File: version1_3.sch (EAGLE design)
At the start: 70 parts, among them U1 LIGHTSA, U2 LIGHTSB, U3 ButtonB, U4 ButtonA

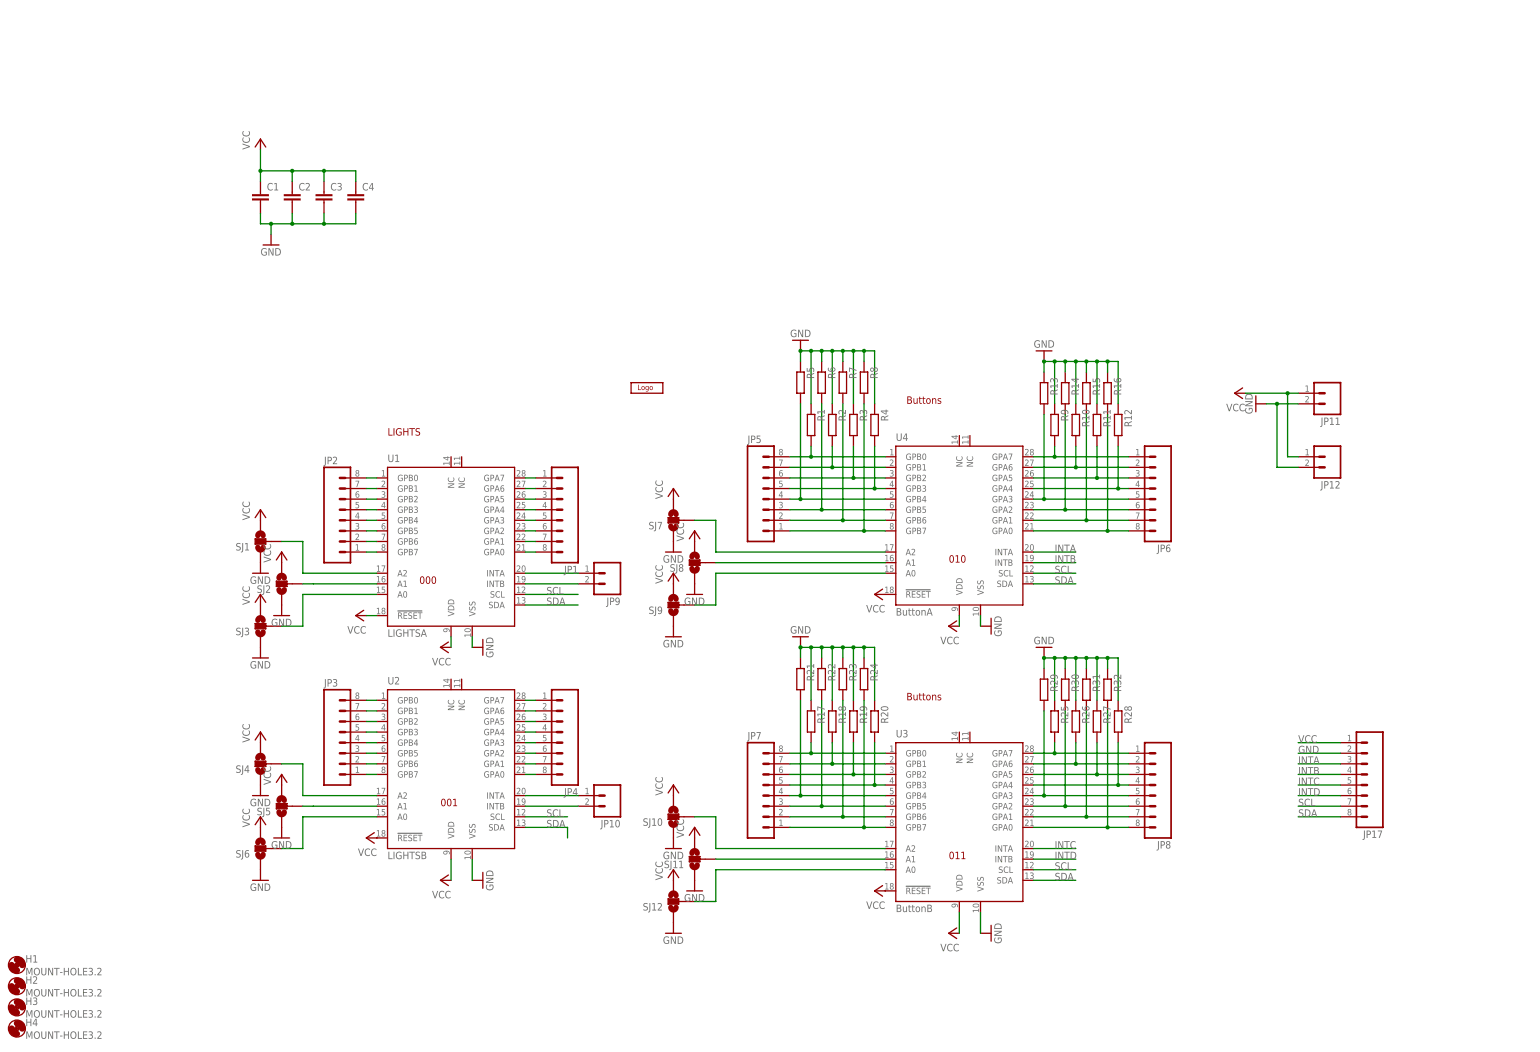
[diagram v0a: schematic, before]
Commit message: folder cleanup and added pdfs and pngs of schematic and layout
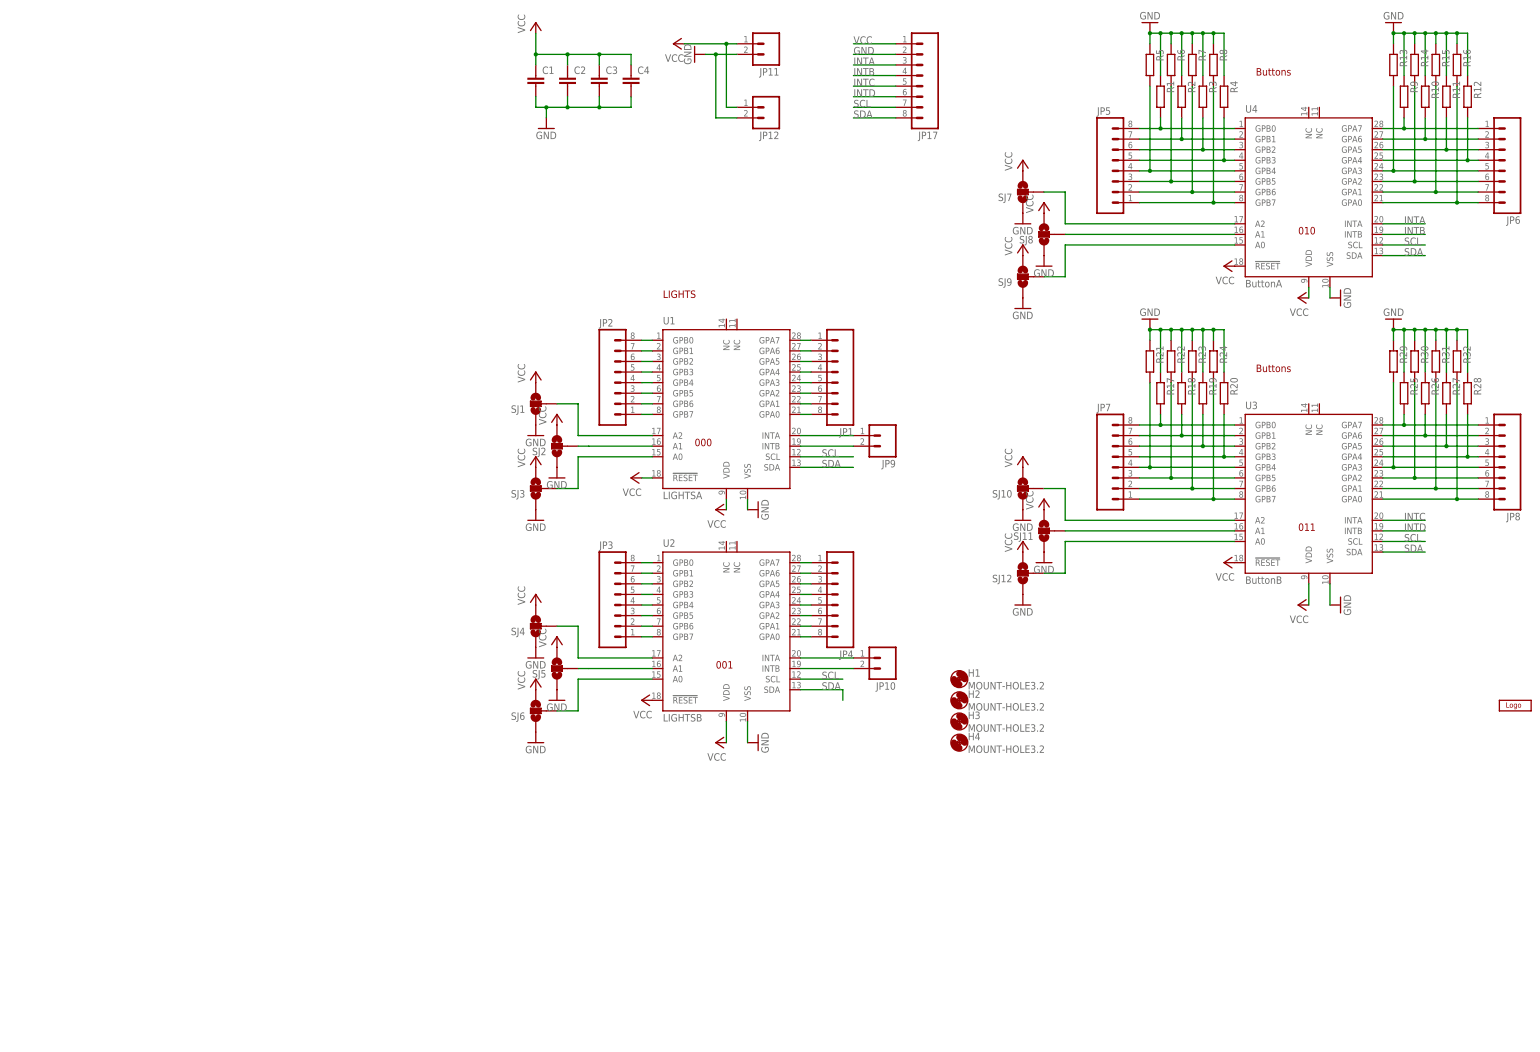
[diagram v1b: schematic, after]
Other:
- moved on the sheet: C1, C2, C3, C4, H1, H2, H3, H4, JP1, JP10, JP11, JP12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
